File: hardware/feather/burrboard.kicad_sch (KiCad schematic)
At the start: 30 parts, among them J1 J1, J2 J2, Q1 TEMT6000X01, U1 TMP36, U2 ADXL345BCCZ

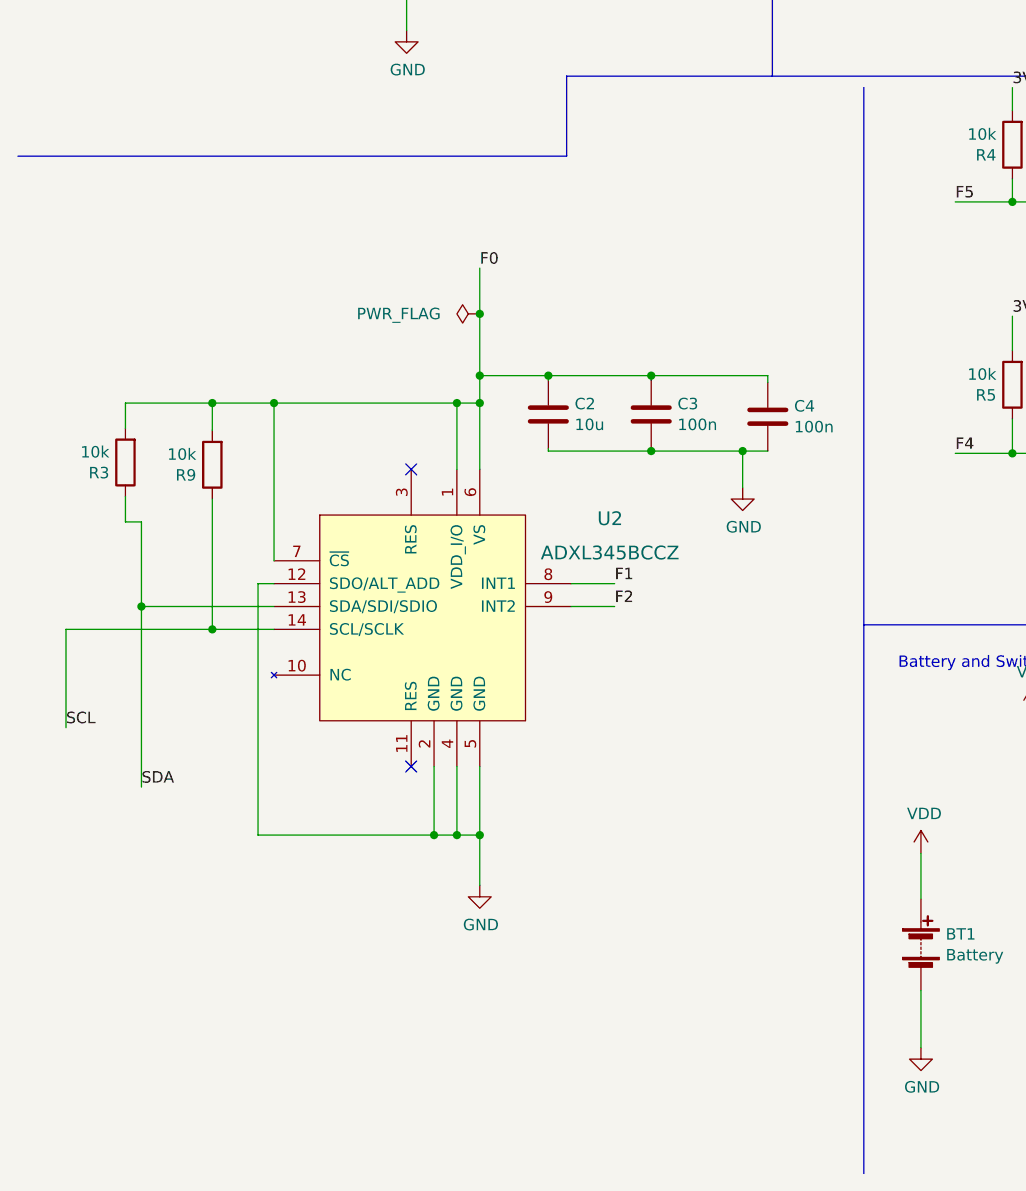
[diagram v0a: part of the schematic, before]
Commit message: Rev 4
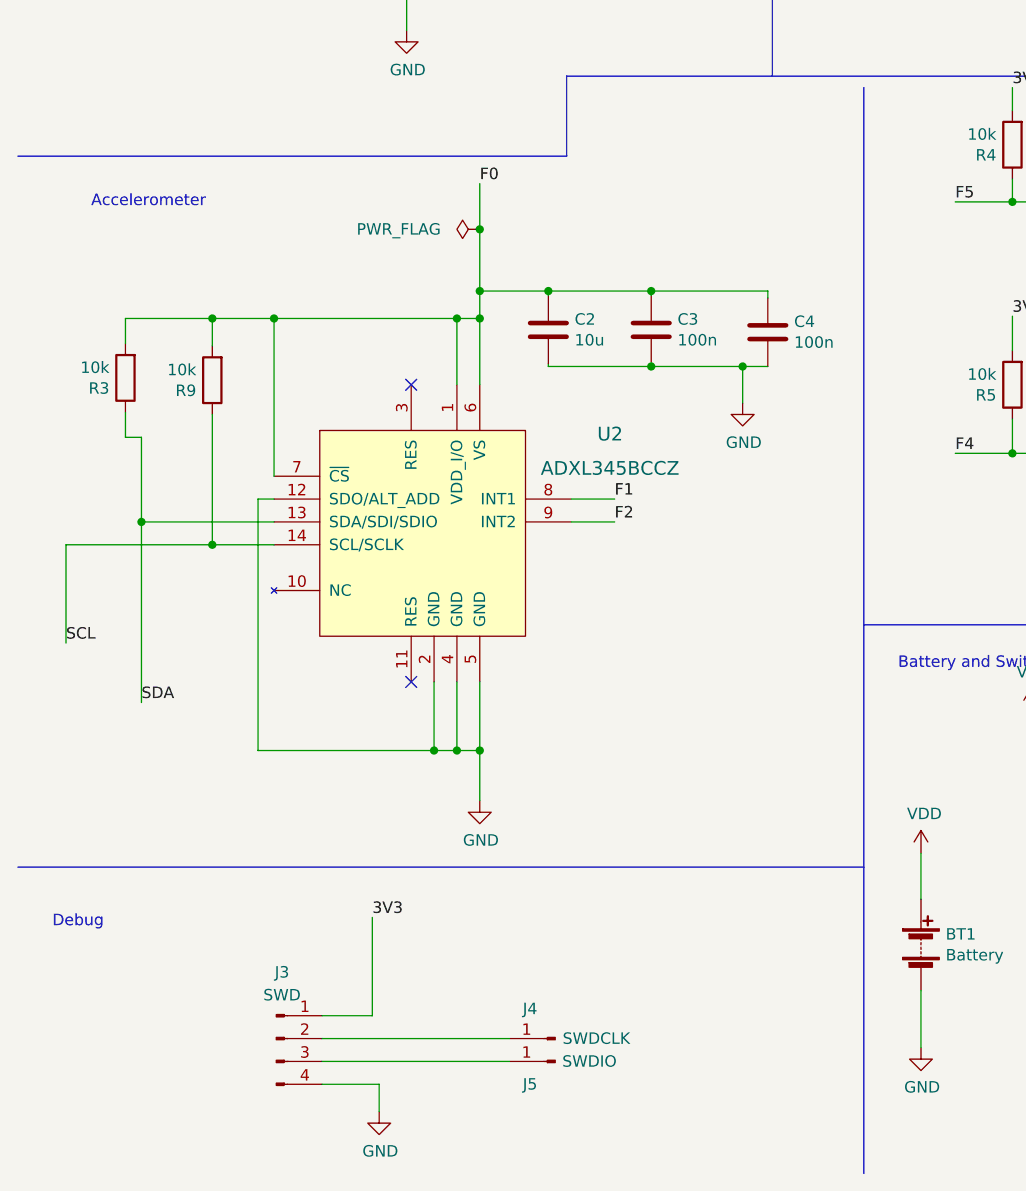
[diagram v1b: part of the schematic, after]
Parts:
- added J3: SWD, Connector_PinHeader_2.54mm:PinHeader_1x04_P2.54mm_Vertical, symbol Connector:Conn_01x04_Male
- added J4: SWDCLK, TestPoint:TestPoint_THTPad_D1.0mm_Drill0.5mm, symbol Connector:Conn_01x01_Male
- added J5: SWDIO, TestPoint:TestPoint_THTPad_D1.0mm_Drill0.5mm, symbol Connector:Conn_01x01_Male
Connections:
- net 3V3: now also J3.1 (Pin_1)
- net GND: now also J3.4 (Pin_4)
- new net: J3.3 (Pin_3), J5.1 (Pin_1)
- new net: J3.2 (Pin_2), J4.1 (Pin_1)
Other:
- note added: "Accelerometer"
- note added: "Debug"
- moved on the sheet: C2, C3, C4, R3, R9, U2

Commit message: Increase size of pogopin footprint
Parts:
- J3: now left out of the parts list
- J4, J5: footprint TestPoint:TestPoint_THTPad_D1.0mm_Drill0.5mm -> TestPoint:TestPoint_THTPad_D1.5mm_Drill0.7mm; now left out of the parts list
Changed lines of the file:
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@@
   )
   (symbol (lib_id "Connector:Conn_01x01_Male") (at 72.39 185.674 180) (unit 1)
-    (in_bom yes) (on_board yes)
+    (in_bom no) (on_board yes)
     (property "Reference" "J5" (id 0) (at 69.596 188.214 0))
     (property "Value" "SWDIO" (id 1) (at 76.2 185.674 0))
-    (property "Footprint" "TestPoint:TestPoint_THTPad_D1.0mm_Drill0.5mm" (id 2) (at 72.39 185.674 0)
+    (property "Footprint" "TestPoint:TestPoint_THTPad_D1.5mm_Drill0.7mm" (id 2) (at 72.39 185.674 0)
       (effects (font (size 1.27 1.27)) hide)
     )
@@
   )
   (symbol (lib_id "Connector:Conn_01x04_Male") (at 41.402 183.134 0) (unit 1)
-    (in_bom yes) (on_board yes) (fields_autoplaced)
+    (in_bom no) (on_board yes) (fields_autoplaced)
     (property "Reference" "J3" (id 0) (at 42.037 175.768 0))
     (property "Value" "SWD" (id 1) (at 42.037 178.308 0))
@@
   )
   (symbol (lib_id "Connector:Conn_01x01_Male") (at 72.39 183.134 180) (unit 1)
-    (in_bom yes) (on_board yes)
+    (in_bom no) (on_board yes)
     (property "Reference" "J4" (id 0) (at 69.596 179.832 0))
     (property "Value" "SWDCLK" (id 1) (at 76.962 183.134 0))
-    (property "Footprint" "TestPoint:TestPoint_THTPad_D1.0mm_Drill0.5mm" (id 2) (at 72.39 183.134 0)
+    (property "Footprint" "TestPoint:TestPoint_THTPad_D1.5mm_Drill0.7mm" (id 2) (at 72.39 183.134 0)
       (effects (font (size 1.27 1.27)) hide)
     )
@@
     )
     (path "/d063ba46-22f6-4e50-9d5e-95f13fbaf268"
-      (reference "J4") (unit 1) (value "SWDCLK") (footprint "TestPoint:TestPoint_THTPad_D1.0mm_Drill0.5mm")
+      (reference "J4") (unit 1) (value "SWDCLK") (footprint "TestPoint:TestPoint_THTPad_D1.5mm_Drill0.7mm")
     )
     (path "/cba8ab97-0377-43bd-bef7-6314ce99d4ae"
-      (reference "J5") (unit 1) (value "SWDIO") (footprint "TestPoint:TestPoint_THTPad_D1.0mm_Drill0.5mm")
+      (reference "J5") (unit 1) (value "SWDIO") (footprint "TestPoint:TestPoint_THTPad_D1.5mm_Drill0.7mm")
     )
     (path "/666dc925-2b95-4de4-a148-45e51fb4be3f"

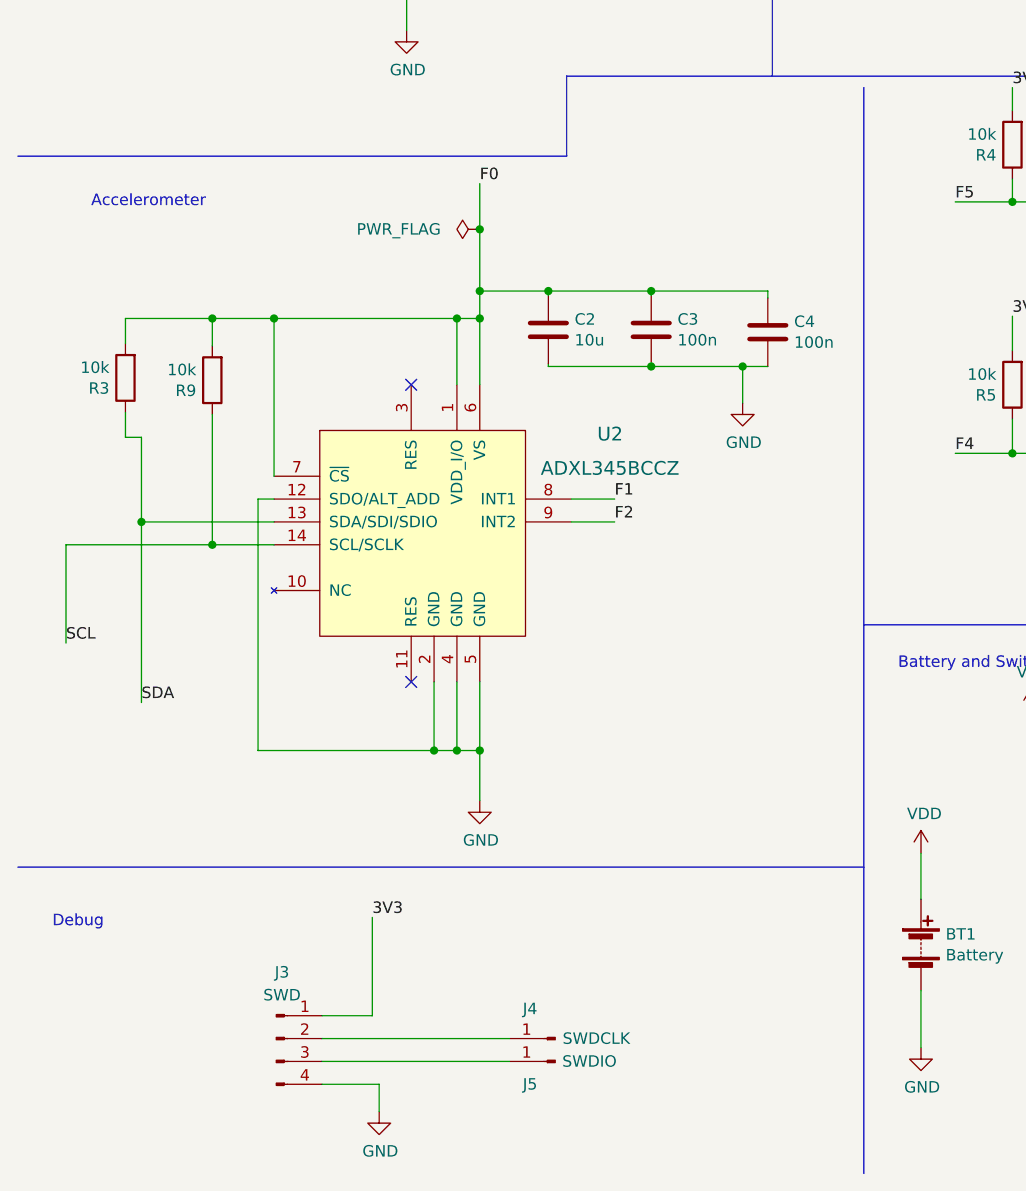
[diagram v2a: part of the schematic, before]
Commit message: Make rev 3.5 final version
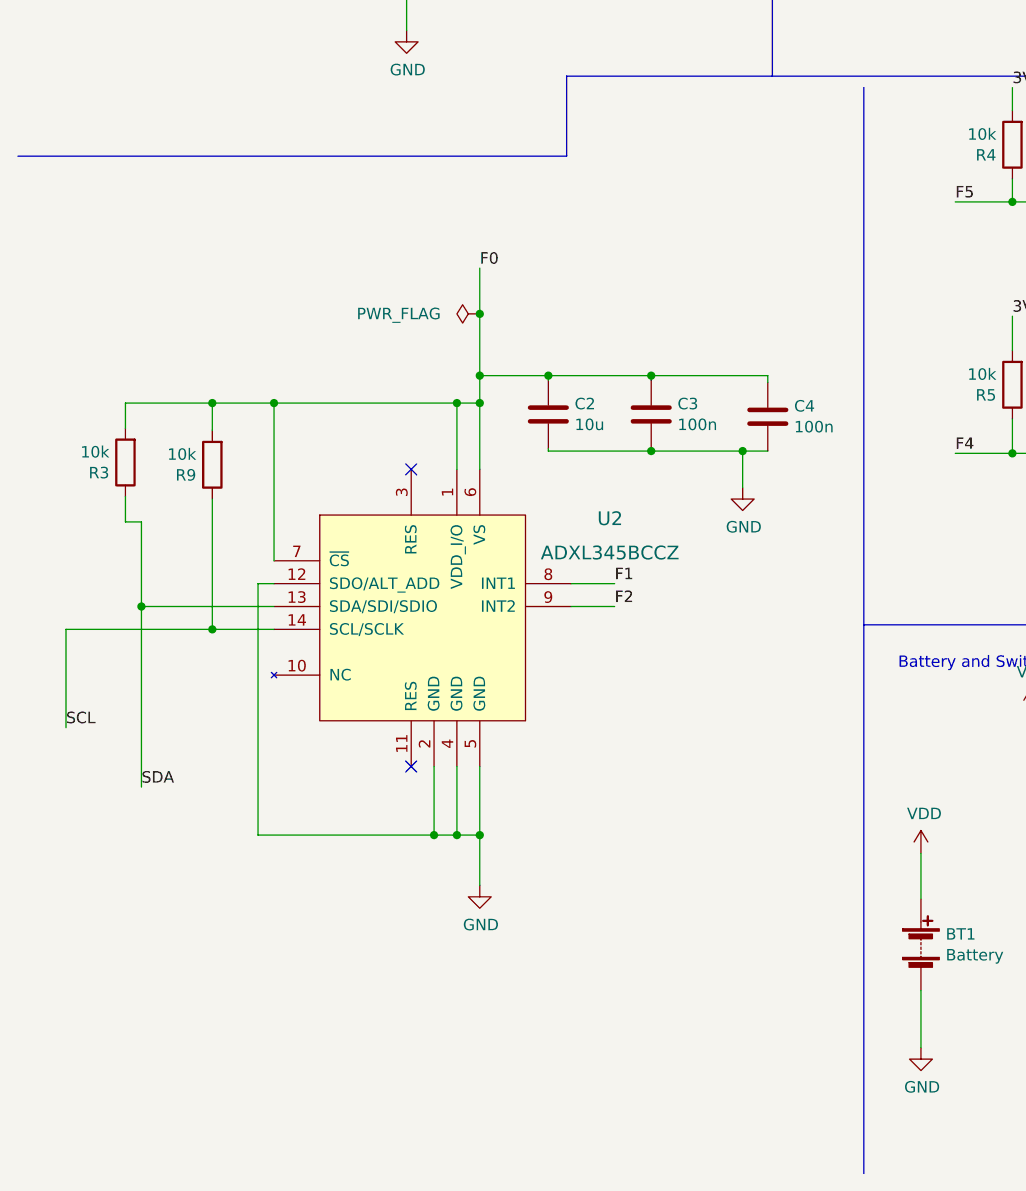
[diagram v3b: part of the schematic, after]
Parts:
- removed J3: SWD, Connector_PinHeader_2.54mm:PinHeader_1x04_P2.54mm_Vertical, symbol Connector:Conn_01x04_Male
- removed J4: SWDCLK, TestPoint:TestPoint_THTPad_D1.5mm_Drill0.7mm, symbol Connector:Conn_01x01_Male
- removed J5: SWDIO, TestPoint:TestPoint_THTPad_D1.5mm_Drill0.7mm, symbol Connector:Conn_01x01_Male
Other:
- note removed: "Accelerometer"
- note removed: "Debug"
- moved on the sheet: C2, C3, C4, R3, R9, U2
